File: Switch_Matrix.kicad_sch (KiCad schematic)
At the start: 146 parts, among them SW1 SW_Push_45deg, SW10 SW_Push_45deg, SW11 SW_Push_45deg, SW12 SW_Push_45deg, SW12(2)1 SW_Push_45deg, SW13 SW_Push_45deg, SW14 SW_Push_45deg, SW15 SW_Push_45deg, SW16 SW_Push_45deg, SW17 SW_Push_45deg, SW18 SW_Push_45deg, SW19 SW_Push_45deg, SW2 SW_Push_45deg, SW20 SW_Push_45deg, SW21 SW_Push_45deg, SW22 SW_Push_45deg, SW23 SW_Push_45deg, SW24 SW_Push_45deg, SW24(1.5)1 SW_Push_45deg, SW25 SW_Push_45deg, SW26 SW_Push_45deg, SW26(2)1 SW_Push_45deg, SW26(ISO)1 SW_Push_45deg, SW27(1.25)1 SW_Push_45deg, SW27(1.5)1 SW_Push_45deg, SW27(ortho)1 SW_Push_45deg, SW28 SW_Push_45deg, SW28(1.5stagger)1 SW_Push_45deg, SW28(ortho)1 SW_Push_45deg, SW29 SW_Push_45deg, SW29(1.5stagger)1 SW_Push_45deg, SW29(ortho)1 SW_Push_45deg, SW3 SW_Push_45deg, SW30 SW_Push_45deg, SW30(1.5stagger)1 SW_Push_45deg, SW30(ortho)1 SW_Push_45deg, SW31 SW_Push_45deg, SW31(1.5stagger)1 SW_Push_45deg, SW31(ortho)1 SW_Push_45deg, SW32 SW_Push_45deg, SW32(1.5stagger)1 SW_Push_45deg, SW32(ortho)1 SW_Push_45deg, SW33 SW_Push_45deg, SW33(1.5stagger)1 SW_Push_45deg, SW33(ortho)1 SW_Push_45deg, SW34 SW_Push_45deg, SW34(1.5stagger)1 SW_Push_45deg, SW34(ortho)1 SW_Push_45deg, SW35 SW_Push_45deg, SW35(1.5stagger)1 SW_Push_45deg, SW35(ortho)1 SW_Push_45deg, SW36 SW_Push_45deg, SW36(1.5stagger)1 SW_Push_45deg, SW36(ortho)1 SW_Push_45deg, SW37 SW_Push_45deg, SW37(1.5stagger)1 SW_Push_45deg, SW37(ortho)1 SW_Push_45deg, SW38(1.25)1 SW_Push_45deg, SW38(1.5)1 SW_Push_45deg, SW38(ortho)1 SW_Push_45deg, SW39 SW_Push_45deg, SW39(1.5)1 SW_Push_45deg, SW4 SW_Push_45deg, SW40 SW_Push_45deg, SW40(3)1 SW_Push_45deg, SW41 SW_Push_45deg, SW41(1.5)1 SW_Push_45deg, SW42(1.25)1 SW_Push_45deg, SW42(1.5)1 SW_Push_45deg, SW42(3)1 SW_Push_45deg, SW43(1.75)1 SW_Push_45deg, SW43(2)1 SW_Push_45deg, SW44(3)1 SW_Push_45deg, SW44(4)1 SW_Push_45deg, SW44(6)1 SW_Push_45deg, SW45(1.75)1 SW_Push_45deg, SW45(2)1 SW_Push_45deg, SW46(1.25)1 SW_Push_45deg, SW46(1.5)1 SW_Push_45deg, SW46(3)1 SW_Push_45deg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

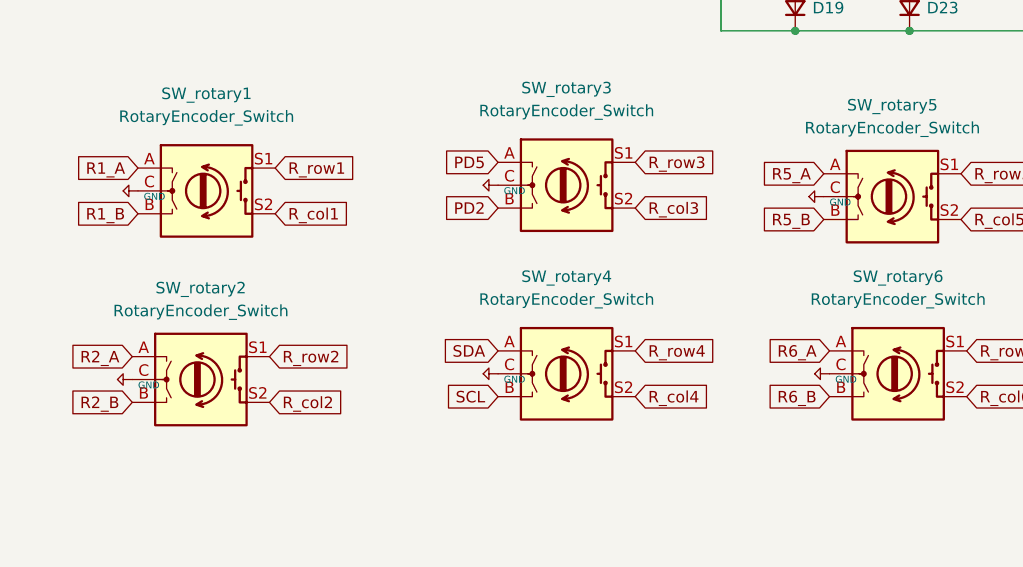
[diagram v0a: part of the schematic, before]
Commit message: encoder, plate
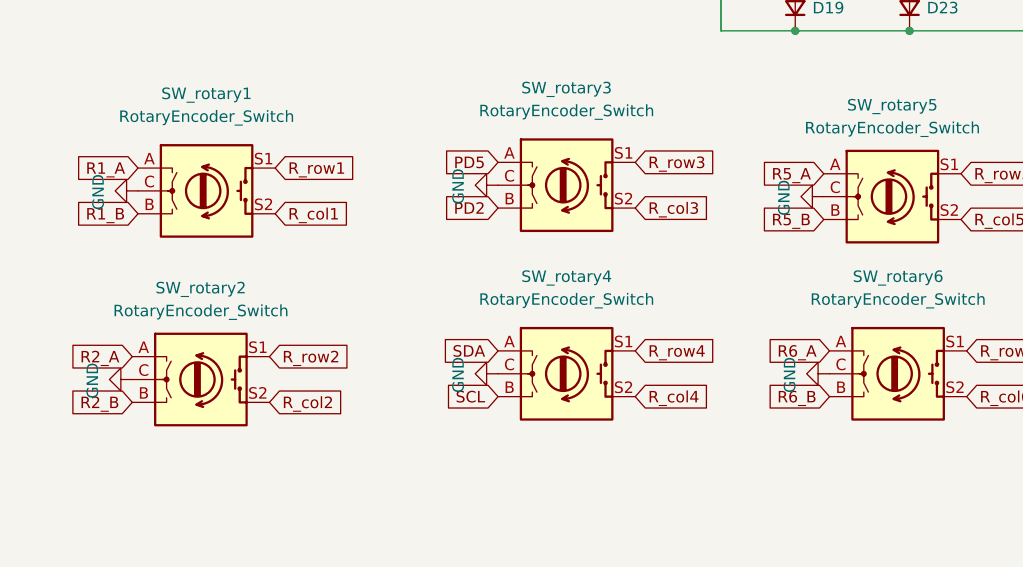
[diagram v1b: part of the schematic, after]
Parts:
- SW_rotary1, SW_rotary2, SW_rotary3, SW_rotary4, SW_rotary5, SW_rotary6: footprint Keebio-Parts:RotaryEncoder_EC11-no-legs -> Keebio-Parts:RotaryEncoder_EC11_Nonplated
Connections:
- net +5V renamed GND
